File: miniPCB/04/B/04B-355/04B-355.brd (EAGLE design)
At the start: 32 parts

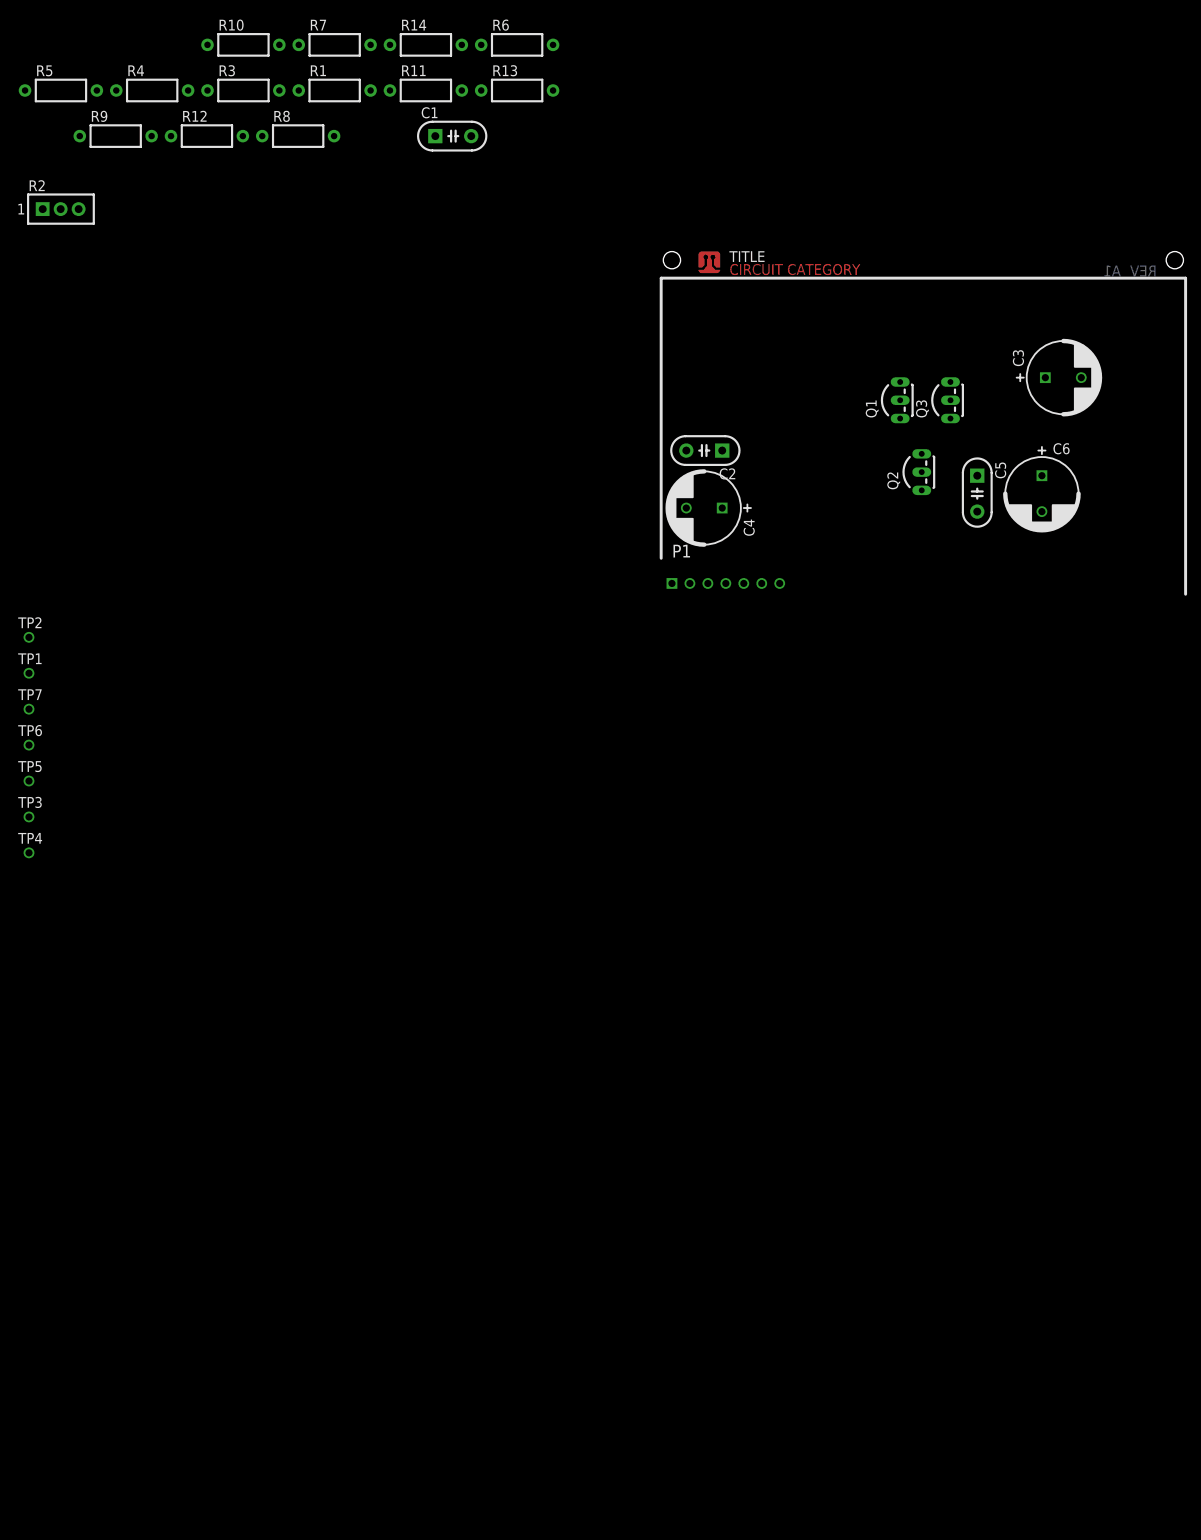
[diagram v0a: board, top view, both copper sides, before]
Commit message: Attempting to fix my Git merge error.
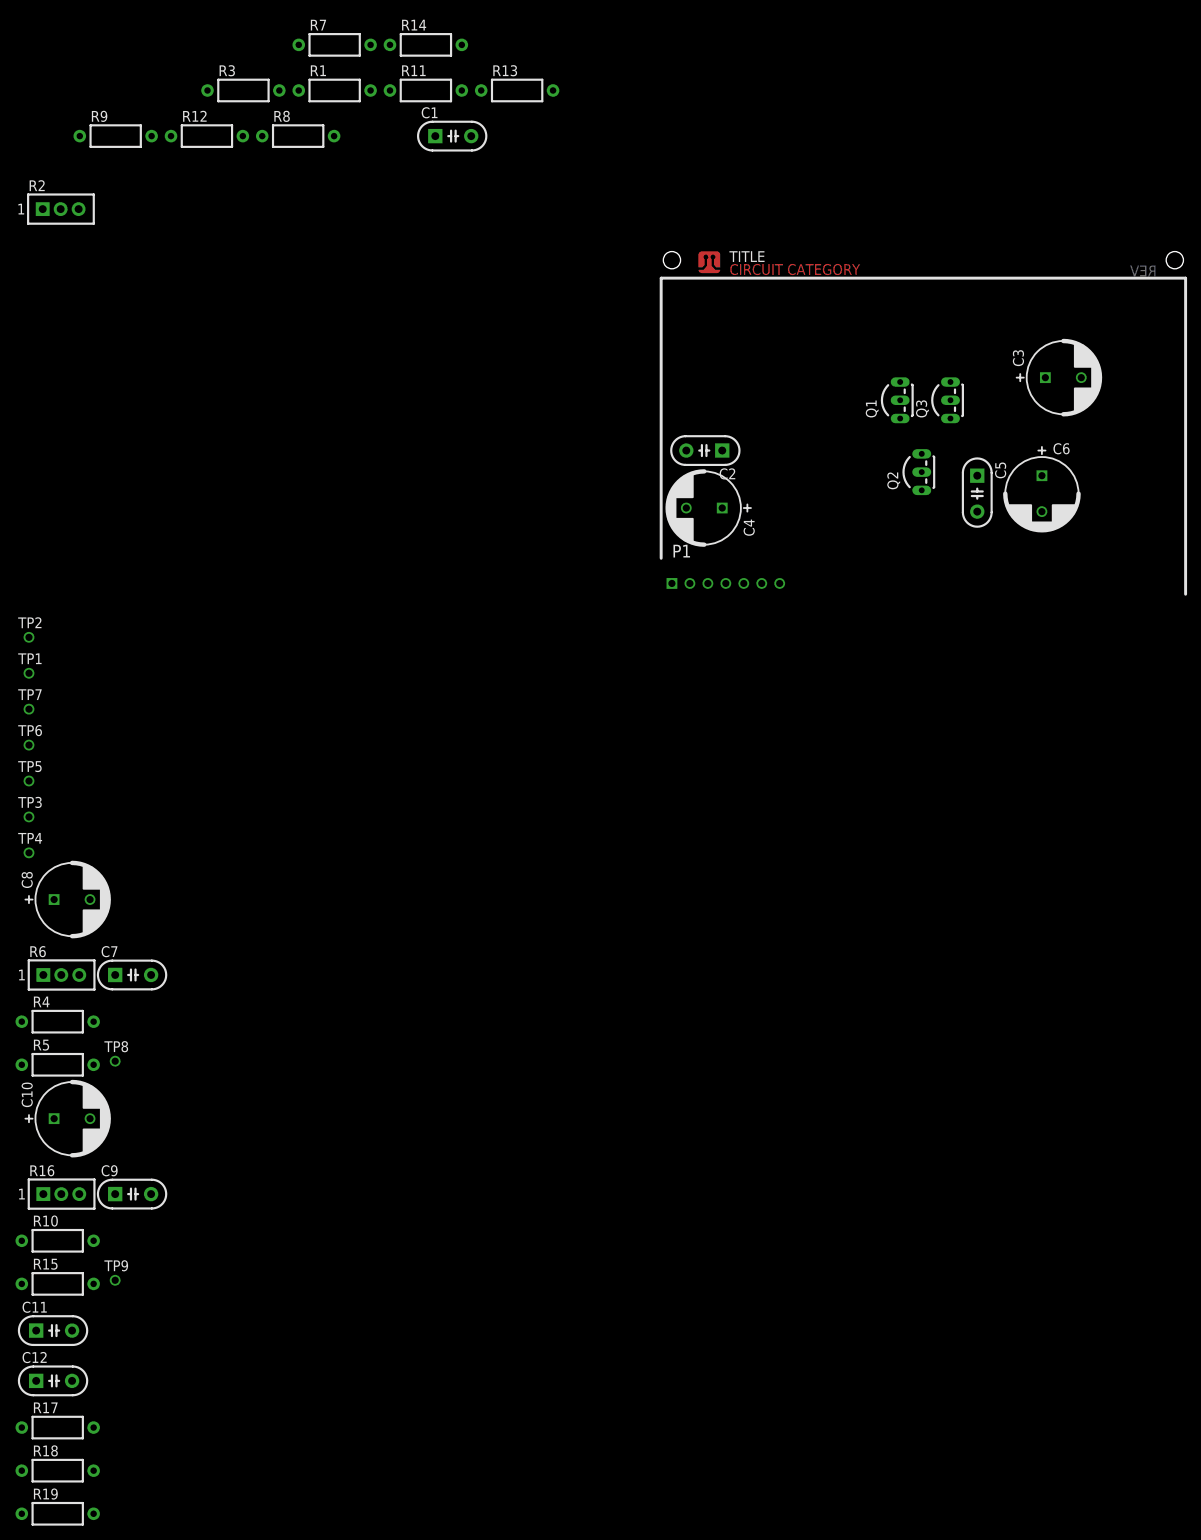
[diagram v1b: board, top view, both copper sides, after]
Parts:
- added C10, C8: (no value), minipcb:C5MM
- added C11, C12, C7, C9: (no value), minipcb:C050-024X044
- added R15, R17, R18, R19: (no value), minipcb:0204/10
- added R16: (no value), minipcb:TRIM_0100
- added TP8, TP9: (no value), minipcb:PINS_1_TESTPOINT_KE5000_NOTEXT
- R6: device minipcb:0204/10 -> minipcb:TRIM_0100
- moved R10 168.5 mm to (-83.0, -89.0)
- moved R6 145.3 mm to (-85.0, -52.0)
- moved R5 135.6 mm to (-83.0, -64.5)
- moved R4 130.3 mm to (-83.0, -58.5)
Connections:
- new net N$15: R4.1, R6.3
- new net N$16: R5.2, R6.1
- new net N$17: C7.1, C8.+, R18.1, R6.2, TP8.1
- new net N$18: R10.1, R16.3
- new net N$19: R15.2, R16.1
- new net N$20: C10.+, C9.1, R16.2, R19.1, TP9.1
- new net N$21: C11.1, P1.5, TP2.1
- new net N$22: C12.1, P1.4, TP1.1
- net GND: now also C10.-, C7.2, C8.-, C9.2, R15.1, R5.1; no longer R10.1
- net N$12: no longer R10.2, R6.1
- net N$14: now also R17.1; no longer R4.2, R5.2, R6.2
- net N$8: now also C12.2; no longer P1.4, R4.1, TP1.1
- net N$9: now also C11.2; no longer P1.5, R5.1, TP2.1
- net V+: now also R10.2, R4.2

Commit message: Attempting to fix my Git merge error.
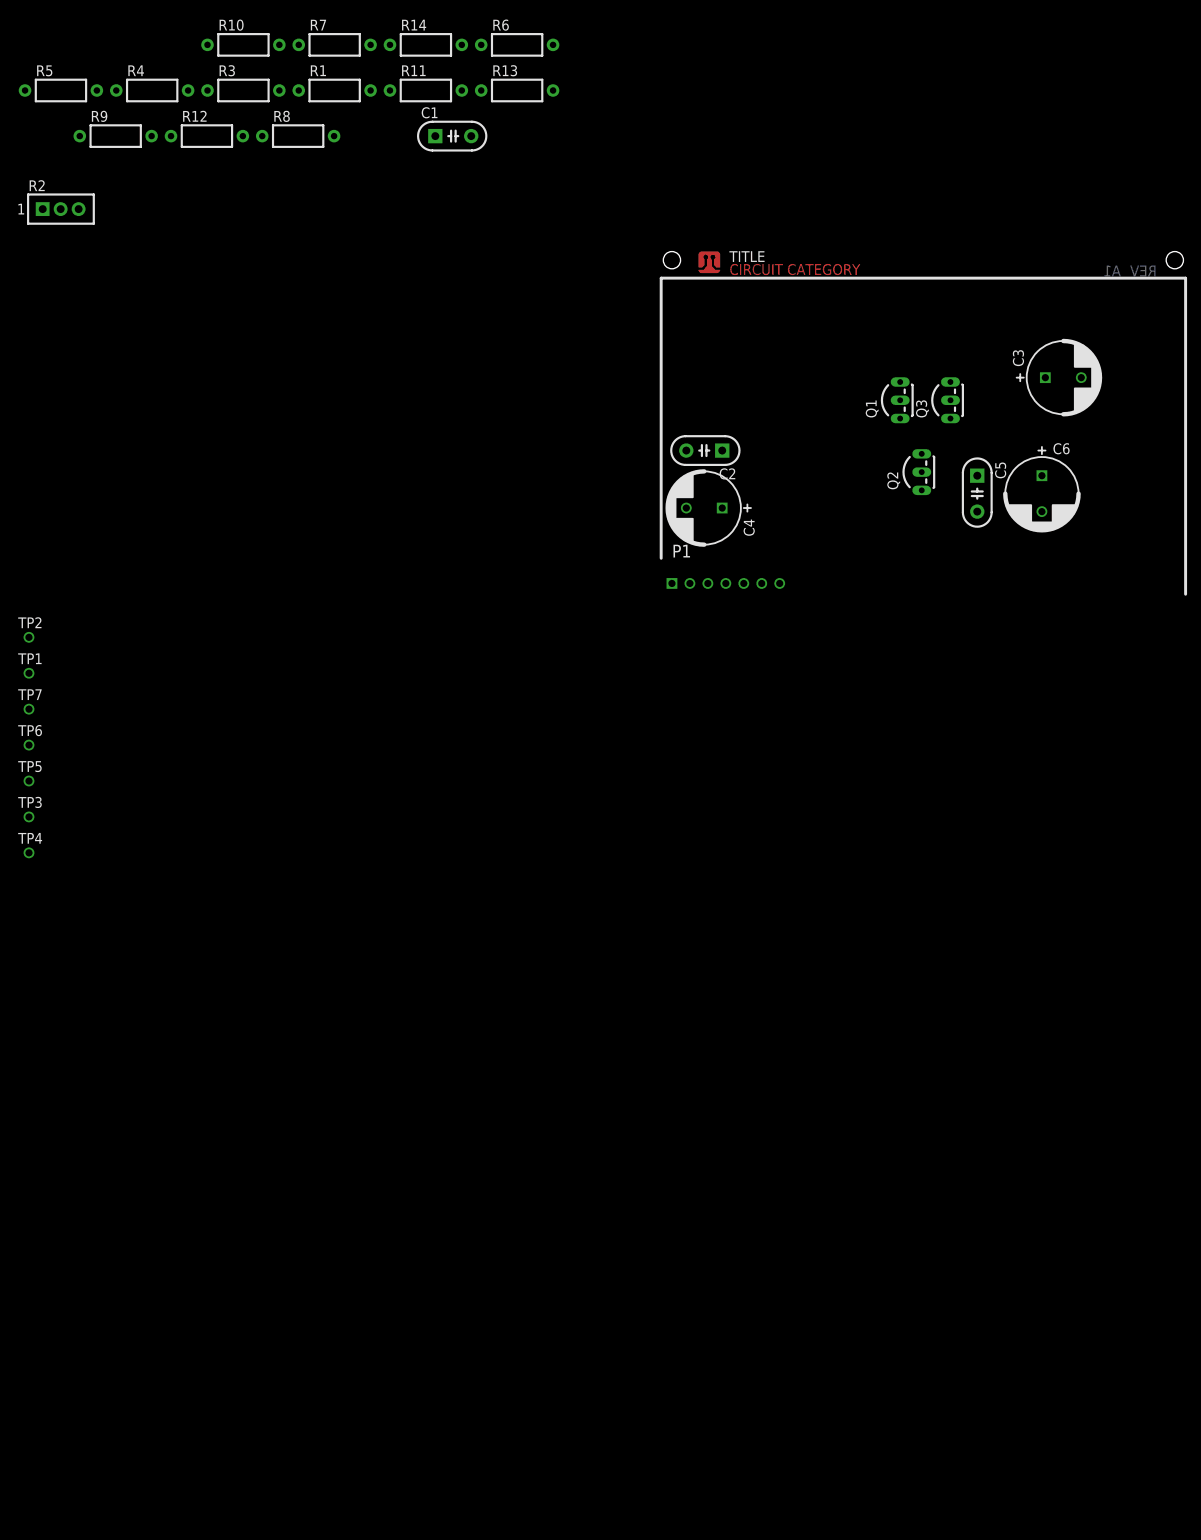
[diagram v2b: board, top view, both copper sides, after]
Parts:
- removed C10, C8: (no value), minipcb:C5MM
- removed C11, C12, C7, C9: (no value), minipcb:C050-024X044
- removed R15, R17, R18, R19: (no value), minipcb:0204/10
- removed R16: (no value), minipcb:TRIM_0100
- removed TP8, TP9: (no value), minipcb:PINS_1_TESTPOINT_KE5000_NOTEXT
- R6: device minipcb:TRIM_0100 -> minipcb:0204/10
- moved R10 168.5 mm to (-57.1, 77.5)
- moved R6 145.3 mm to (-19.1, 77.5)
- moved R5 135.6 mm to (-82.5, 71.1)
- moved R4 130.3 mm to (-69.8, 71.1)
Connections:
- removed net N$15: R4.1, R6.3
- removed net N$16: R5.2, R6.1
- removed net N$17: C7.1, C8.+, R18.1, R6.2, TP8.1
- removed net N$18: R10.1, R16.3
- removed net N$19: R15.2, R16.1
- removed net N$20: C10.+, C9.1, R16.2, R19.1, TP9.1
- removed net N$21: C11.1, P1.5, TP2.1
- removed net N$22: C12.1, P1.4, TP1.1
- net GND: now also R10.1; no longer C10.-, C7.2, C8.-, C9.2, R15.1, R5.1
- net N$12: now also R10.2, R6.1
- net N$14: now also R4.2, R5.2, R6.2; no longer R17.1
- net N$8: now also P1.4, R4.1, TP1.1; no longer C12.2
- net N$9: now also P1.5, R5.1, TP2.1; no longer C11.2
- net V+: no longer R10.2, R4.2
